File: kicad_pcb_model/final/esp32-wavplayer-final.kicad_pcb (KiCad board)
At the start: 2 copper layers, 32 x 63.8 mm, 0 parts

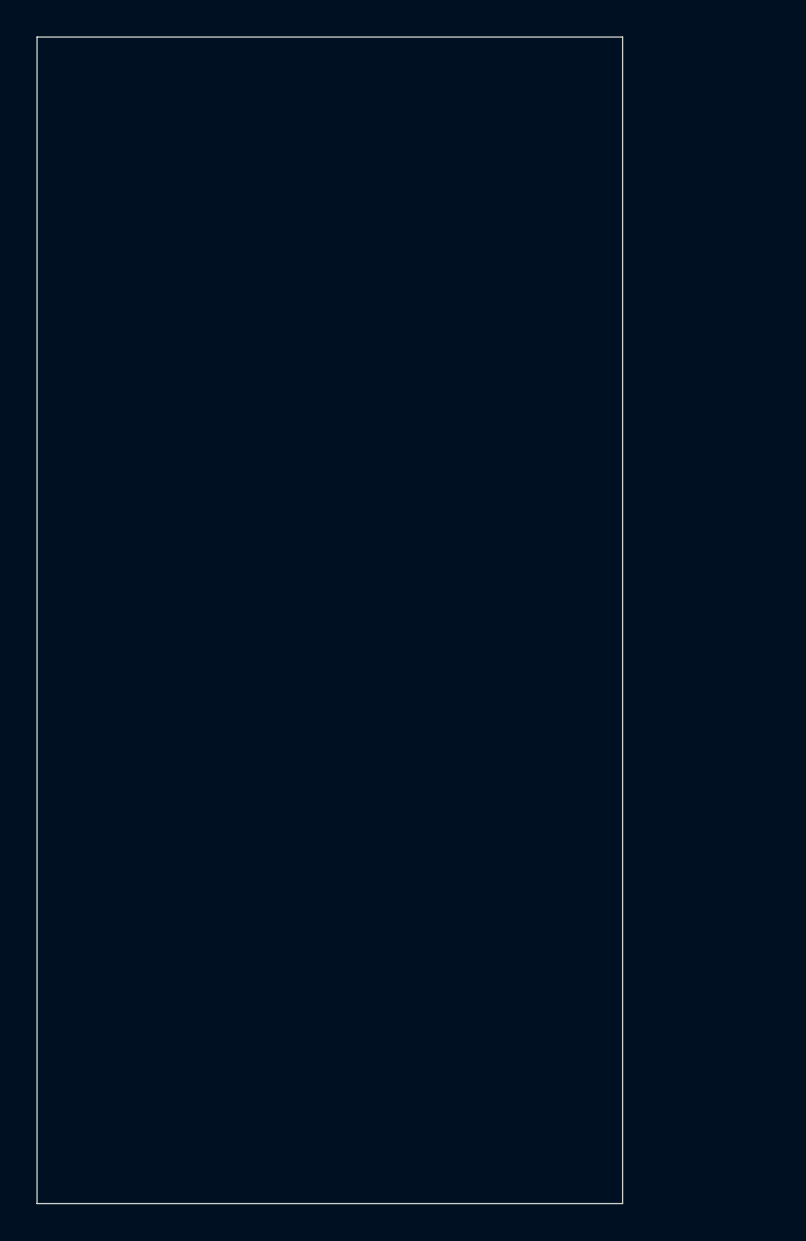
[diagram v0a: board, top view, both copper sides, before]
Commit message: updated wisevision configuration
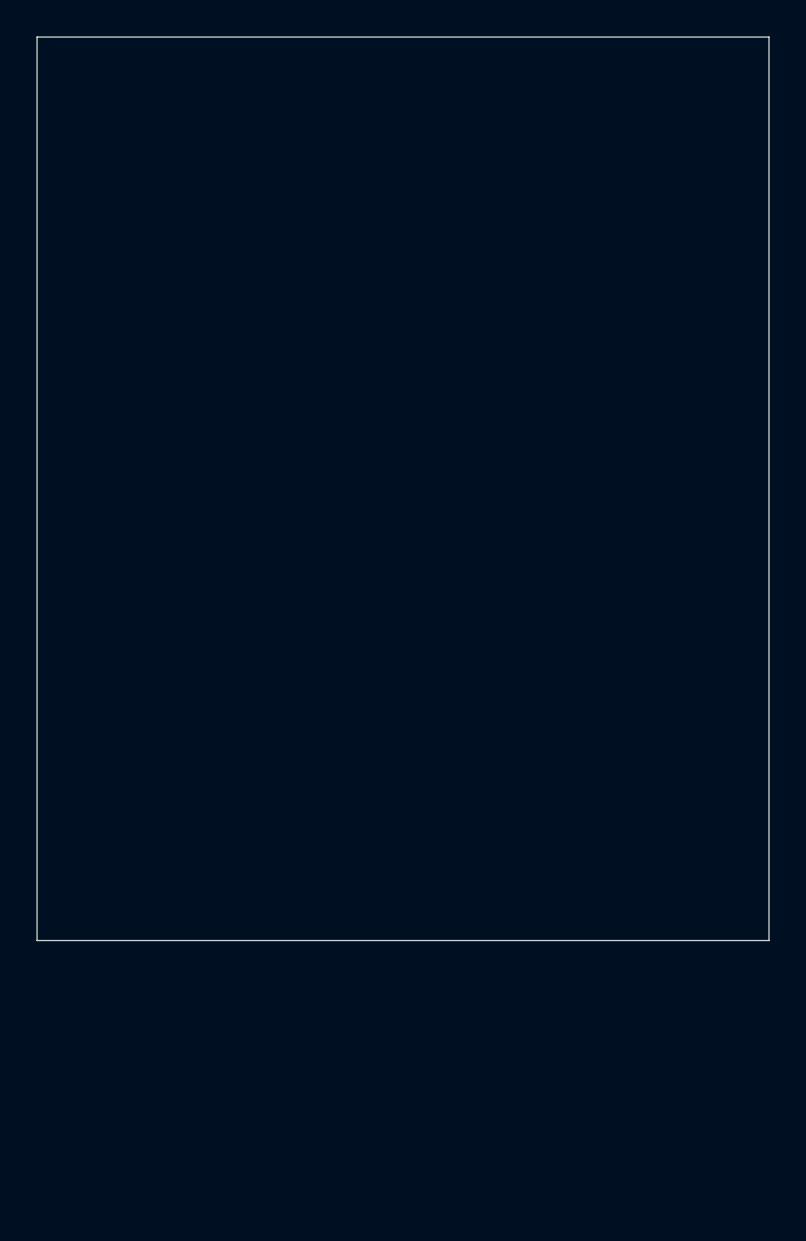
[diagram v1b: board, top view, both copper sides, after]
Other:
- board size 32 x 63.8 mm -> 40 x 49.4 mm
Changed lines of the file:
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@@
 	(gr_rect
 		(start 134.25 69.875)
-		(end 166.25 133.625)
+		(end 174.25 119.25)
 		(stroke
 			(width 0.05)

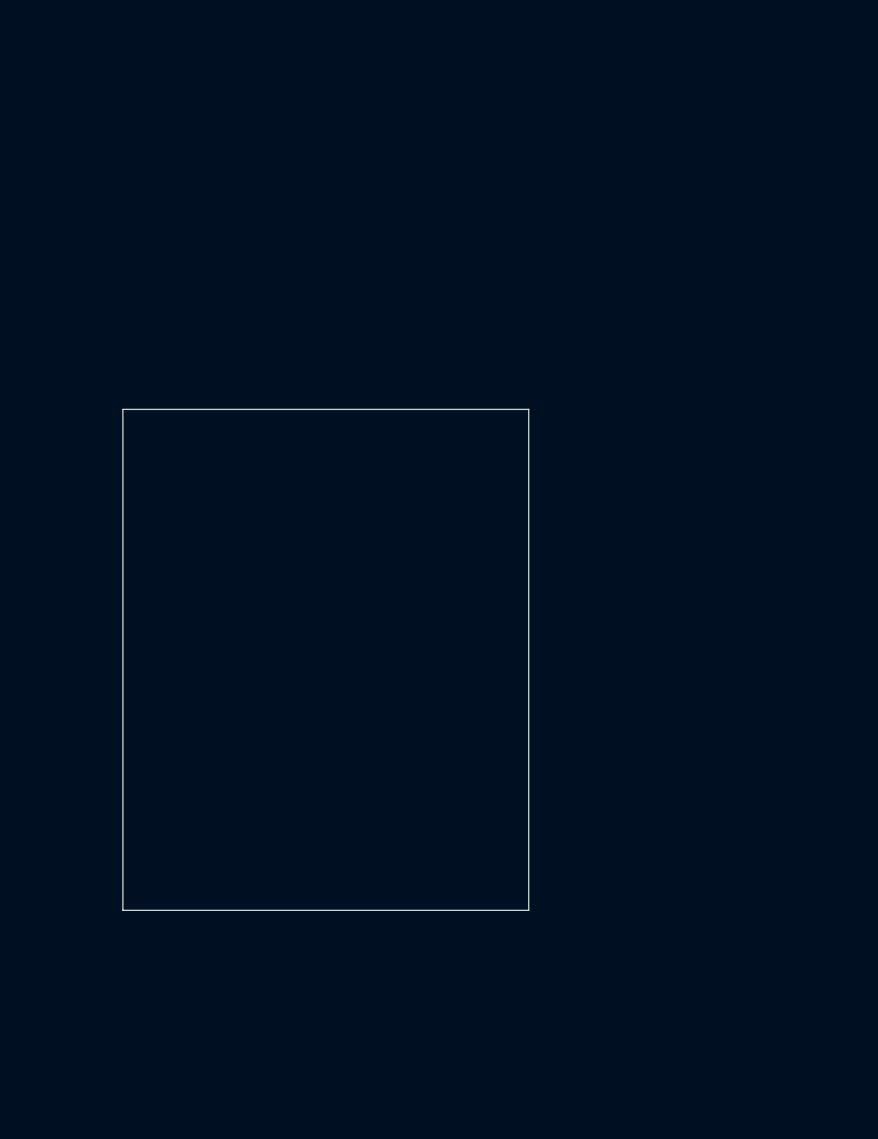
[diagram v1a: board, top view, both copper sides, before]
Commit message: updating model
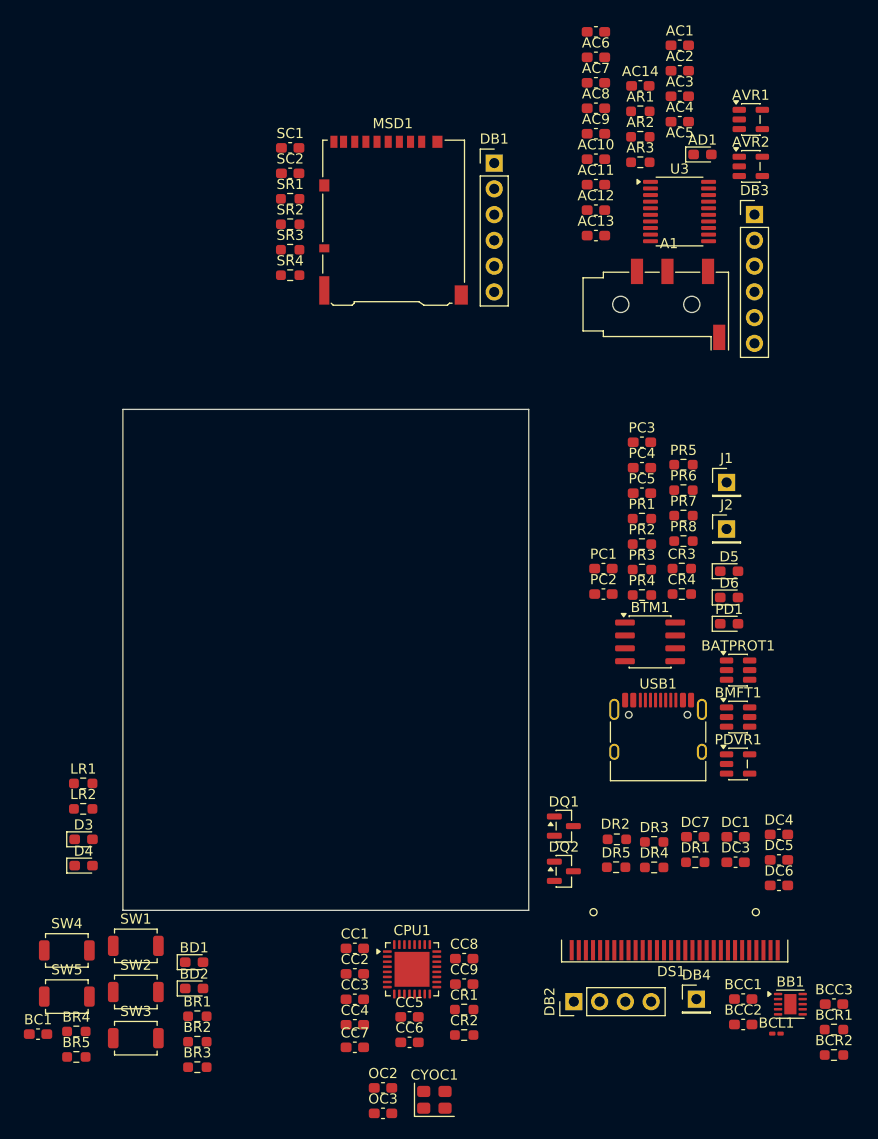
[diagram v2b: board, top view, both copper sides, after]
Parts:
- added A1: 3.5mmAudioJack, Connector_Audio:Jack_3.5mm_KoreanHropartsElec_PJ-320D-4A_Horizontal, F.Cu at (188.1, 59.5)
- added AC1: 0.1uF, Capacitor_SMD:C_0603_1608Metric_Pad1.08x0.95mm_HandSolder, F.Cu at (189.1, 34.0)
- added AC10: 0.1uF, Capacitor_SMD:C_0603_1608Metric_Pad1.08x0.95mm_HandSolder, F.Cu at (180.9, 45.2)
- added AC11: 2.2uF, Capacitor_SMD:C_0603_1608Metric_Pad1.08x0.95mm_HandSolder, F.Cu at (180.9, 47.7)
- added AC12: 2.2nF, Capacitor_SMD:C_0603_1608Metric_Pad1.08x0.95mm_HandSolder, F.Cu at (180.9, 50.2)
- added AC13: 2.2nF, Capacitor_SMD:C_0603_1608Metric_Pad1.08x0.95mm_HandSolder, F.Cu at (180.9, 52.7)
- added AC14: 2.2uF, Capacitor_SMD:C_0603_1608Metric_Pad1.08x0.95mm_HandSolder, F.Cu at (185.2, 38.0)
- added AC2: 10uF, Capacitor_SMD:C_0603_1608Metric_Pad1.08x0.95mm_HandSolder, F.Cu at (189.1, 36.5)
- added AC3: 0.1uF, Capacitor_SMD:C_0603_1608Metric_Pad1.08x0.95mm_HandSolder, F.Cu at (189.1, 39.0)
- added AC4: 0.1uF, Capacitor_SMD:C_0603_1608Metric_Pad1.08x0.95mm_HandSolder, F.Cu at (189.1, 41.5)
- added AC5: 10uF, Capacitor_SMD:C_0603_1608Metric_Pad1.08x0.95mm_HandSolder, F.Cu at (180.9, 32.7)
- added AC6: 0.1uF, Capacitor_SMD:C_0603_1608Metric_Pad1.08x0.95mm_HandSolder, F.Cu at (180.9, 35.2)
- added AC7: 10uF, Capacitor_SMD:C_0603_1608Metric_Pad1.08x0.95mm_HandSolder, F.Cu at (180.9, 37.7)
- added AC8: 0.1uF, Capacitor_SMD:C_0603_1608Metric_Pad1.08x0.95mm_HandSolder, F.Cu at (180.9, 40.2)
- added AC9: 10uF, Capacitor_SMD:C_0603_1608Metric_Pad1.08x0.95mm_HandSolder, F.Cu at (180.9, 42.7)
- added AD1: D, Diode_SMD:D_0603_1608Metric_Pad1.05x0.95mm_HandSolder, F.Cu at (191.4, 44.8)
- added AR1: 470, Resistor_SMD:R_0603_1608Metric_Pad0.98x0.95mm_HandSolder, F.Cu at (185.2, 40.5)
- added AR2: 470, Resistor_SMD:R_0603_1608Metric_Pad0.98x0.95mm_HandSolder, F.Cu at (185.2, 43.0)
- added AR3: 1k, Resistor_SMD:R_0603_1608Metric_Pad0.98x0.95mm_HandSolder, F.Cu at (185.2, 45.5)
- added AVR1: ME6211C33M5, Package_TO_SOT_SMD:SOT-23-5, F.Cu at (196.1, 41.3)
- added AVR2: ME6211C33M5, Package_TO_SOT_SMD:SOT-23-5, F.Cu at (196.1, 45.9)
- added BATPROT1: DW01A, Package_TO_SOT_SMD:SOT-23-6, F.Cu at (194.9, 95.6)
- added BB1: TPS63030DSK, Package_SON:WSON-10-1EP_2.5x2.5mm_P0.5mm_EP1.2x2mm, F.Cu at (200.0, 128.5)
- added BC1: 100nF, Capacitor_SMD:C_0603_1608Metric_Pad1.08x0.95mm_HandSolder, F.Cu at (125.9, 131.4)
- added BCC1: 0.1uF, Capacitor_SMD:C_0603_1608Metric_Pad1.08x0.95mm_HandSolder, F.Cu at (195.4, 128.0)
- added BCC2: 10uF, Capacitor_SMD:C_0603_1608Metric_Pad1.08x0.95mm_HandSolder, F.Cu at (195.4, 130.5)
- added BCC3: 10uF, Capacitor_SMD:C_0603_1608Metric_Pad1.08x0.95mm_HandSolder, F.Cu at (204.3, 128.5)
- added BCL1: 2.2uH, Inductor_SMD:L_0201_0603Metric_Pad0.64x0.40mm_HandSolder, F.Cu at (198.7, 131.4)
- added BCR1: 200k, Resistor_SMD:R_0603_1608Metric_Pad0.98x0.95mm_HandSolder, F.Cu at (204.3, 131.0)
- added BCR2: 1.2M, Resistor_SMD:R_0603_1608Metric_Pad0.98x0.95mm_HandSolder, F.Cu at (204.3, 133.5)
- added BD1: D, Diode_SMD:D_0603_1608Metric_Pad1.05x0.95mm_HandSolder, F.Cu at (141.3, 124.4)
- added BD2: D, Diode_SMD:D_0603_1608Metric_Pad1.05x0.95mm_HandSolder, F.Cu at (141.3, 127.0)
- added BMFT1: FS8205A, Package_TO_SOT_SMD:SOT-23-6, F.Cu at (194.9, 100.2)
- added BR1: 10k, Resistor_SMD:R_0603_1608Metric_Pad0.98x0.95mm_HandSolder, F.Cu at (141.6, 129.7)
- added BR2: 10k, Resistor_SMD:R_0603_1608Metric_Pad0.98x0.95mm_HandSolder, F.Cu at (141.6, 132.2)
- added BR3: 4.7k, Resistor_SMD:R_0603_1608Metric_Pad0.98x0.95mm_HandSolder, F.Cu at (141.6, 134.7)
- added BR4: 6.8k, Resistor_SMD:R_0603_1608Metric_Pad0.98x0.95mm_HandSolder, F.Cu at (129.7, 131.2)
- added BR5: 15k, Resistor_SMD:R_0603_1608Metric_Pad0.98x0.95mm_HandSolder, F.Cu at (129.7, 133.7)
- added BTM1: TP4056-42-ESOP8, Package_SO:SOIC-8_3.9x4.9mm_P1.27mm, F.Cu at (186.2, 92.8)
- added CC1: 1uF, Capacitor_SMD:C_0603_1608Metric_Pad1.08x0.95mm_HandSolder, F.Cu at (157.1, 123.0)
- added CC2: 1uF, Capacitor_SMD:C_0603_1608Metric_Pad1.08x0.95mm_HandSolder, F.Cu at (157.1, 125.5)
- added CC3: 100nF, Capacitor_SMD:C_0603_1608Metric_Pad1.08x0.95mm_HandSolder, F.Cu at (157.1, 128.0)
- added CC4: 100nF, Capacitor_SMD:C_0603_1608Metric_Pad1.08x0.95mm_HandSolder, F.Cu at (157.1, 130.5)
- added CC5: 1uF, Capacitor_SMD:C_0603_1608Metric_Pad1.08x0.95mm_HandSolder, F.Cu at (162.5, 129.8)
- added CC6: 10uF, Capacitor_SMD:C_0603_1608Metric_Pad1.08x0.95mm_HandSolder, F.Cu at (162.5, 132.3)
- added CC7: 1uF, Capacitor_SMD:C_0603_1608Metric_Pad1.08x0.95mm_HandSolder, F.Cu at (157.1, 132.8)
- added CC8: 10nF, Capacitor_SMD:C_0603_1608Metric_Pad1.08x0.95mm_HandSolder, F.Cu at (167.9, 124.0)
- added CC9: 10nF, Capacitor_SMD:C_0603_1608Metric_Pad1.08x0.95mm_HandSolder, F.Cu at (167.9, 126.5)
- added CPU1: ESP32-C3-H*, Package_DFN_QFN:QFN-32-1EP_5x5mm_P0.5mm_EP3.45x3.45mm, F.Cu at (162.8, 125.1)
- added CR1: 10k, Resistor_SMD:R_0603_1608Metric_Pad0.98x0.95mm_HandSolder, F.Cu at (167.9, 129.0)
- added CR2: 10k, Resistor_SMD:R_0603_1608Metric_Pad0.98x0.95mm_HandSolder, F.Cu at (167.9, 131.5)
- added CR3: 22R, Resistor_SMD:R_0603_1608Metric_Pad0.98x0.95mm_HandSolder, F.Cu at (189.3, 85.6)
- added CR4: 22R, Resistor_SMD:R_0603_1608Metric_Pad0.98x0.95mm_HandSolder, F.Cu at (189.3, 88.1)
- added CYOC1: 3225-40m, Oscillator:Oscillator_SMD_Abracon_ASE-4Pin_3.2x2.5mm, F.Cu at (164.9, 137.9)
- added D3: PWRLED, LED_SMD:LED_0603_1608Metric_Pad1.05x0.95mm_HandSolder, F.Cu at (130.4, 112.2)
- added D4: ONLED, LED_SMD:LED_0603_1608Metric_Pad1.05x0.95mm_HandSolder, F.Cu at (130.4, 114.8)
- added D5: CHRGLED, LED_SMD:LED_0603_1608Metric_Pad1.05x0.95mm_HandSolder, F.Cu at (194.0, 85.8)
- added D6: STNDLED, LED_SMD:LED_0603_1608Metric_Pad1.05x0.95mm_HandSolder, F.Cu at (194.0, 88.4)
- added DB1: MicroSDDebug, Connector_PinHeader_2.54mm:PinHeader_1x06_P2.54mm_Vertical, F.Cu at (170.8, 45.6)
- added DB2: DisplayDebug, Connector_PinHeader_2.54mm:PinHeader_1x04_P2.54mm_Vertical, F.Cu at (178.7, 128.2)
- added DB3: PCM5102aDebug, Connector_PinHeader_2.54mm:PinHeader_1x06_P2.54mm_Vertical, F.Cu at (196.5, 50.7)
- added DB4: DebugPinVbat, Connector_PinHeader_2.54mm:PinHeader_1x01_P2.54mm_Vertical, F.Cu at (190.8, 128.0)
- added DC1: 2.2uF, Capacitor_SMD:C_0603_1608Metric_Pad1.08x0.95mm_HandSolder, F.Cu at (194.6, 112.0)
- added DC3: 1uF, Capacitor_SMD:C_0603_1608Metric_Pad1.08x0.95mm_HandSolder, F.Cu at (194.6, 114.5)
- added DC4: 1uF, Capacitor_SMD:C_0603_1608Metric_Pad1.08x0.95mm_HandSolder, F.Cu at (198.9, 111.8)
- added DC5: 1uF, Capacitor_SMD:C_0603_1608Metric_Pad1.08x0.95mm_HandSolder, F.Cu at (198.9, 114.3)
- added DC6: 1uF, Capacitor_SMD:C_0603_1608Metric_Pad1.08x0.95mm_HandSolder, F.Cu at (198.9, 116.8)
- added DC7: 4.7uF, Capacitor_SMD:C_0603_1608Metric_Pad1.08x0.95mm_HandSolder, F.Cu at (190.7, 112.0)
- added DQ1: FDN338P, Package_TO_SOT_SMD:SOT-23, F.Cu at (177.7, 111.0)
- added DQ2: FDN335N, Package_TO_SOT_SMD:SOT-23, F.Cu at (177.7, 115.4)
- added DR1: 4.7k, Resistor_SMD:R_0603_1608Metric_Pad0.98x0.95mm_HandSolder, F.Cu at (190.7, 114.5)
- added DR2: 4.7k, Resistor_SMD:R_0603_1608Metric_Pad0.98x0.95mm_HandSolder, F.Cu at (182.9, 112.2)
- added DR3: 620k, Resistor_SMD:R_0603_1608Metric_Pad0.98x0.95mm_HandSolder, F.Cu at (186.6, 112.5)
- added DR4: 47k, Resistor_SMD:R_0603_1608Metric_Pad0.98x0.95mm_HandSolder, F.Cu at (186.6, 115.0)
- added DR5: 47k, Resistor_SMD:R_0603_1608Metric_Pad0.98x0.95mm_HandSolder, F.Cu at (182.9, 115.0)
- added DS1: Wisevision X096-2864KSWPG01-H30, Display:OLED-128O064D, F.Cu at (188.6, 123.2)
- added J1: BIN+, Connector_PinHeader_2.54mm:PinHeader_1x01_P2.54mm_Vertical, F.Cu at (193.8, 77.1)
- added J2: BIN-, Connector_PinHeader_2.54mm:PinHeader_1x01_P2.54mm_Vertical, F.Cu at (193.8, 81.7)
- added LR1: 5.1k, Resistor_SMD:R_0603_1608Metric_Pad0.98x0.95mm_HandSolder, F.Cu at (130.3, 106.7)
- added LR2: 5.1k, Resistor_SMD:R_0603_1608Metric_Pad0.98x0.95mm_HandSolder, F.Cu at (130.3, 109.2)
- added MSD1: Generic MicroSD, Connector_Card:microSD_HC_Hirose_DM3AT-SF-PEJM5, F.Cu at (160.9, 51.2)
- added OC2: 15pF, Capacitor_SMD:C_0603_1608Metric_Pad1.08x0.95mm_HandSolder, F.Cu at (159.9, 136.8)
- added OC3: 15pF, Capacitor_SMD:C_0603_1608Metric_Pad1.08x0.95mm_HandSolder, F.Cu at (159.9, 139.3)
- added PC1: 10uF, Capacitor_SMD:C_0603_1608Metric_Pad1.08x0.95mm_HandSolder, F.Cu at (181.6, 85.6)
- added PC2: 10uF, Capacitor_SMD:C_0603_1608Metric_Pad1.08x0.95mm_HandSolder, F.Cu at (181.6, 88.1)
- added PC3: 10uF, Capacitor_SMD:C_0603_1608Metric_Pad1.08x0.95mm_HandSolder, F.Cu at (185.4, 73.1)
- added PC4: 100nF, Capacitor_SMD:C_0603_1608Metric_Pad1.08x0.95mm_HandSolder, F.Cu at (185.4, 75.6)
- added PC5: 10uF, Capacitor_SMD:C_0603_1608Metric_Pad1.08x0.95mm_HandSolder, F.Cu at (185.4, 78.1)
- added PD1: D, Diode_SMD:D_0603_1608Metric_Pad1.05x0.95mm_HandSolder, F.Cu at (194.0, 91.0)
- added PDVR1: ME6211C33M5, Package_TO_SOT_SMD:SOT-23-5, F.Cu at (194.9, 104.8)
- added PR1: 5.1K, Resistor_SMD:R_0603_1608Metric_Pad0.98x0.95mm_HandSolder, F.Cu at (185.4, 80.6)
- added PR2: 5.1K, Resistor_SMD:R_0603_1608Metric_Pad0.98x0.95mm_HandSolder, F.Cu at (185.4, 83.2)
- added PR3: 0.4, Resistor_SMD:R_0603_1608Metric_Pad0.98x0.95mm_HandSolder, F.Cu at (185.4, 85.7)
- added PR4: 1k, Resistor_SMD:R_0603_1608Metric_Pad0.98x0.95mm_HandSolder, F.Cu at (185.4, 88.2)
- added PR5: 1k, Resistor_SMD:R_0603_1608Metric_Pad0.98x0.95mm_HandSolder, F.Cu at (189.5, 75.3)
- added PR6: 1k, Resistor_SMD:R_0603_1608Metric_Pad0.98x0.95mm_HandSolder, F.Cu at (189.5, 77.8)
- added PR7: 100, Resistor_SMD:R_0603_1608Metric_Pad0.98x0.95mm_HandSolder, F.Cu at (189.5, 80.3)
- added PR8: 1K, Resistor_SMD:R_0603_1608Metric_Pad0.98x0.95mm_HandSolder, F.Cu at (189.5, 82.9)
- added SC1: 100nF, Capacitor_SMD:C_0603_1608Metric_Pad1.08x0.95mm_HandSolder, F.Cu at (150.7, 44.1)
- added SC2: 10nF, Capacitor_SMD:C_0603_1608Metric_Pad1.08x0.95mm_HandSolder, F.Cu at (150.7, 46.6)
- added SR1: 10k, Resistor_SMD:R_0603_1608Metric_Pad0.98x0.95mm_HandSolder, F.Cu at (150.7, 49.1)
- added SR2: 10k, Resistor_SMD:R_0603_1608Metric_Pad0.98x0.95mm_HandSolder, F.Cu at (150.7, 51.6)
- added SR3: 10k, Resistor_SMD:R_0603_1608Metric_Pad0.98x0.95mm_HandSolder, F.Cu at (150.7, 54.1)
- added SR4: 10k, Resistor_SMD:R_0603_1608Metric_Pad0.98x0.95mm_HandSolder, F.Cu at (150.7, 56.6)
- added SW1: RST, Button_Switch_SMD:SW_SPST_TS-1088-xR020, F.Cu at (135.5, 122.8)
- added SW2: BOOT/UP, Button_Switch_SMD:SW_SPST_TS-1088-xR020, F.Cu at (135.5, 127.3)
- added SW3: RIGHT, Button_Switch_SMD:SW_SPST_TS-1088-xR020, F.Cu at (135.5, 131.8)
- added SW4: LEFT, Button_Switch_SMD:SW_SPST_TS-1088-xR020, F.Cu at (128.7, 123.2)
- added SW5: DOWN, Button_Switch_SMD:SW_SPST_TS-1088-xR020, F.Cu at (128.7, 127.8)
- added U3: PCM5102A, Package_SO:TSSOP-20_4.4x6.5mm_P0.65mm, F.Cu at (189.1, 50.4)
- added USB1: USBC-6Pin, Connector_USB:USB_C_Receptacle_HRO_TYPE-C-31-M-12, F.Cu at (187.0, 102.6)
